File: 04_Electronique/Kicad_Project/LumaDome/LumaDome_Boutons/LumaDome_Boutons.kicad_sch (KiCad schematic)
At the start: 6 parts, among them J1 Conn_01x03, SW1 SW_Push, SW2 SW_Push, SW3 SW_Push

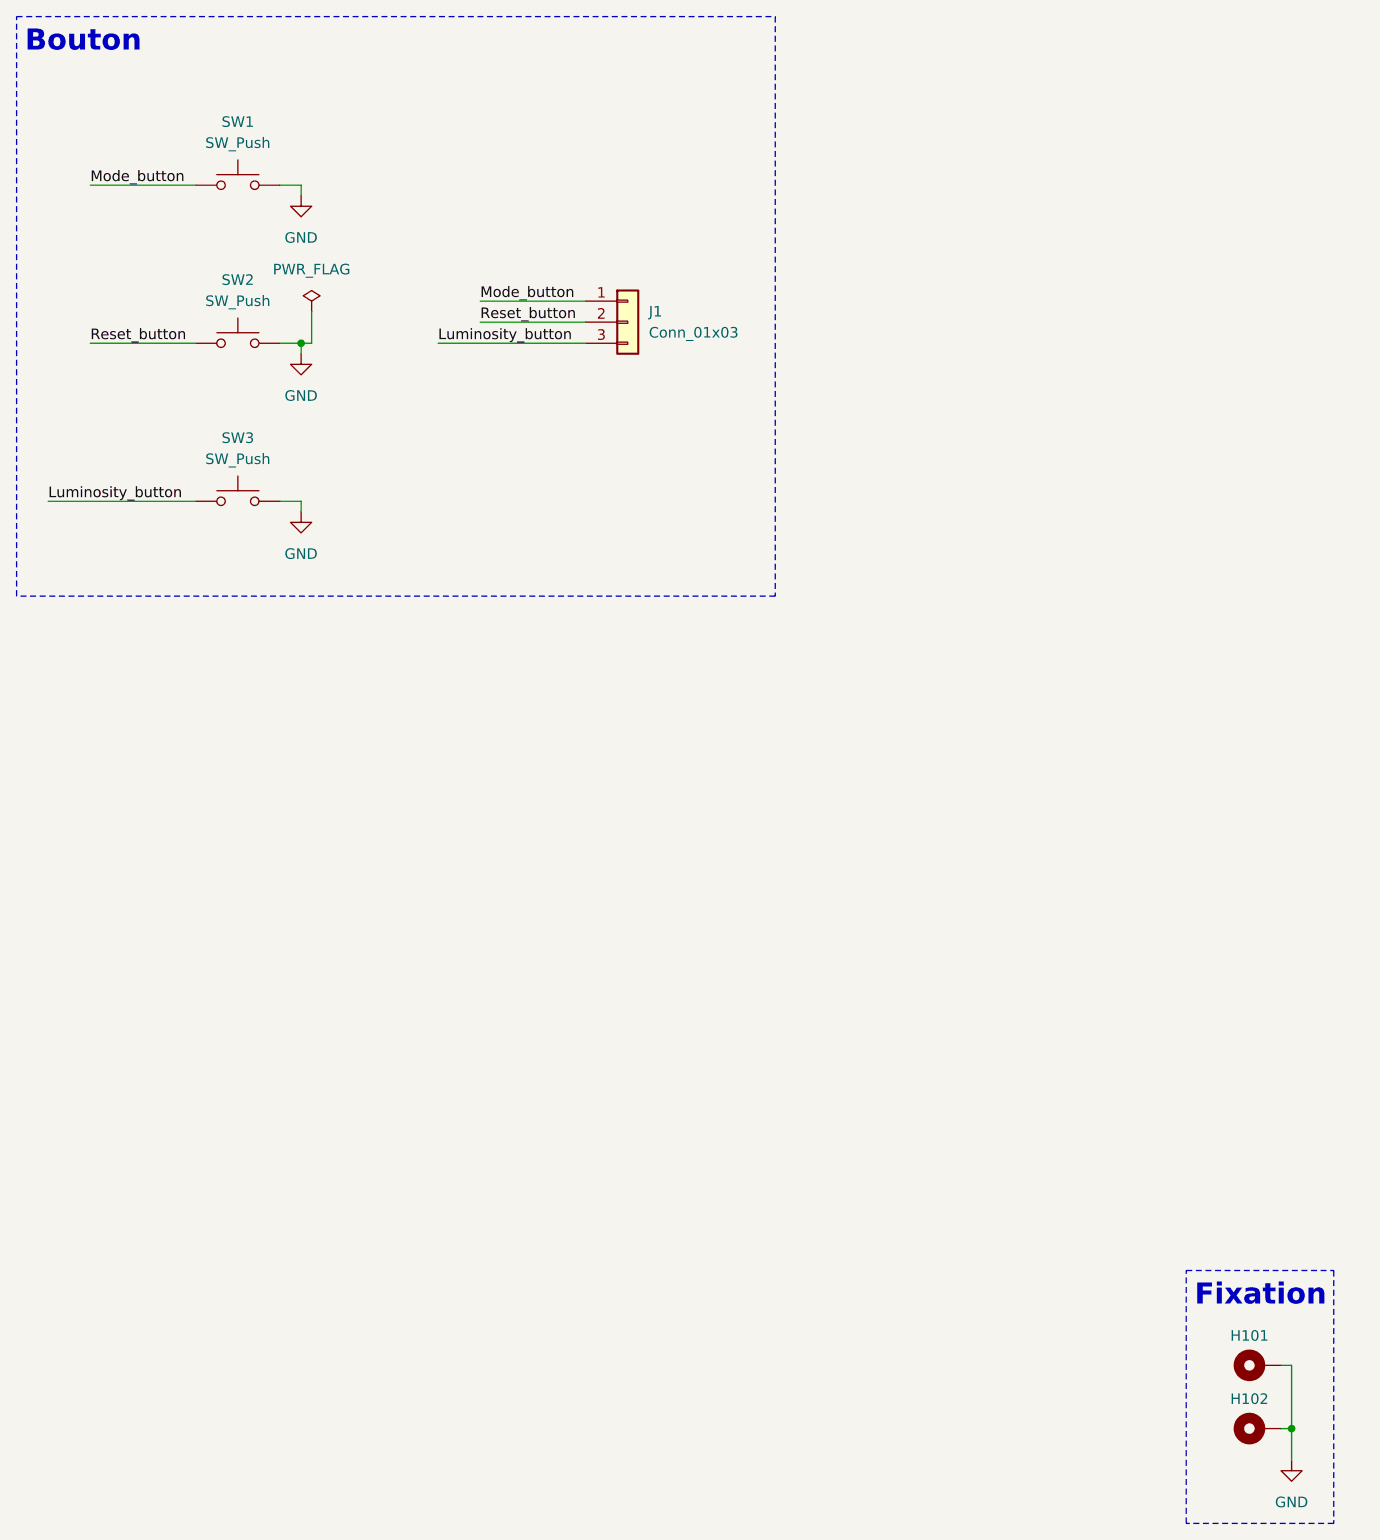
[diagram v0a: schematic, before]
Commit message: Finalisation PCB 02
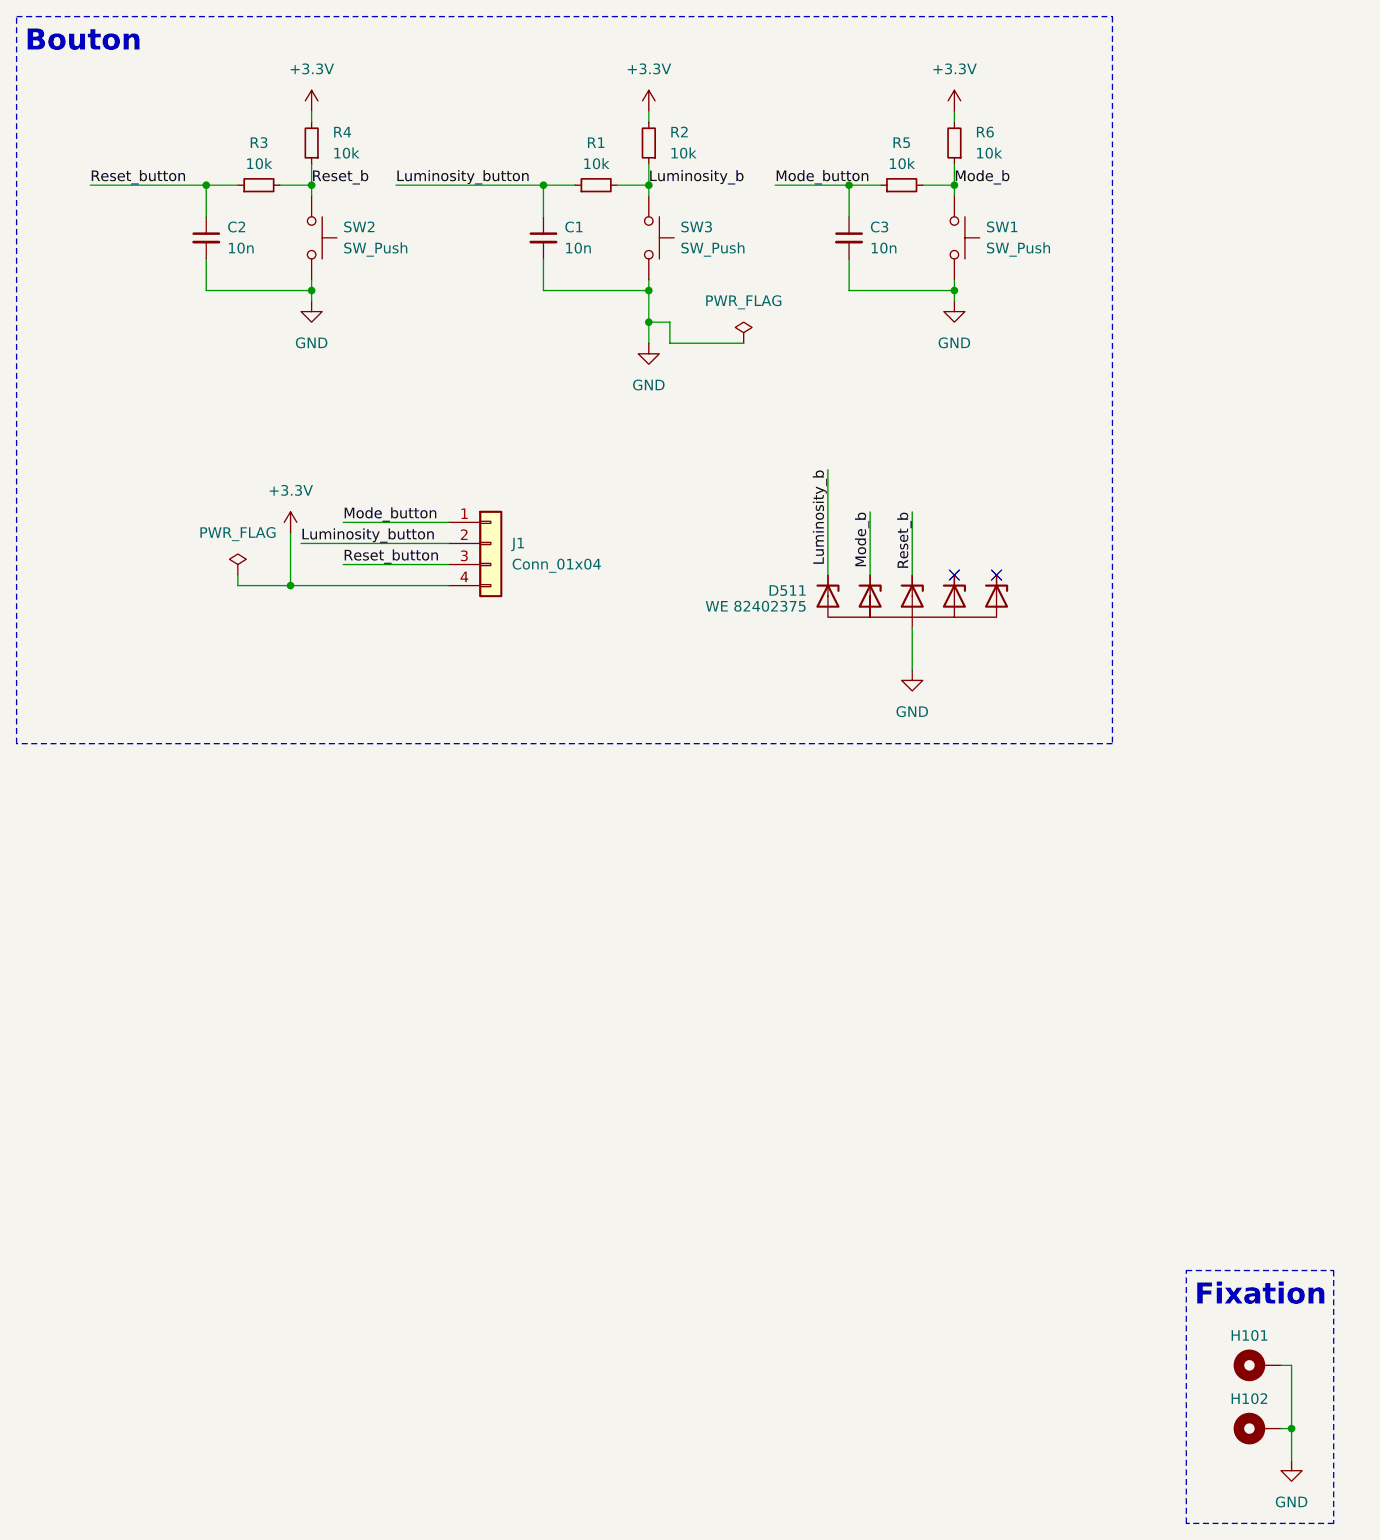
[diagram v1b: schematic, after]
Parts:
- removed J1: Conn_01x03, Connector_PinHeader_1.27mm:PinHeader_1x03_P1.27mm_Vertical, symbol Connector_Generic:Conn_01x03
- added C1, C2, C3: 10n, Capacitor_SMD:C_0402_1005Metric, symbol Device:C_Small
- added D511: WE 82402375, MaximeRempreinte:SC70-6L, symbol mylibs:D_TVS_Uni_x5
- added J1: Conn_01x04, Connector_PinHeader_1.27mm:PinHeader_1x04_P1.27mm_Vertical, symbol Connector_Generic:Conn_01x04
- added R1, R2, R3, R4, R5, R6: 10k, Resistor_SMD:R_0402_1005Metric, symbol Device:R_Small
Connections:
- net GND: now also C1.2, C2.2, C3.2, D511.2 (GND)
- net Luminosity_button: now also C1.1, J1.2 (Pin_2), R1.1; no longer SW3.1
- net Mode_button: now also C3.1, J1.1 (Pin_1), R5.1; no longer SW1.1
- net Reset_button: now also C2.1, J1.3 (Pin_3), R3.1; no longer SW2.1
- new net +3.3V: J1.4 (Pin_4), R2.2, R4.2, R6.2
- new net Luminosity_b: D511.6 (I/O), R1.2, R2.1, SW3.1
- new net Mode_b: D511.5 (I/O), R5.2, R6.1, SW1.1
- new net Reset_b: D511.4 (I/O), R3.2, R4.1, SW2.1
- no-connect marks 0 -> 2
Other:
- moved on the sheet: SW1
